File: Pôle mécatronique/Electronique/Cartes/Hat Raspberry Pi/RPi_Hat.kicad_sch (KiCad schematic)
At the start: 9 parts, among them J1 Conn_02x03_Odd_Even, U1 XBee, U2 MCP25625-x-SS, Y1 8MHz

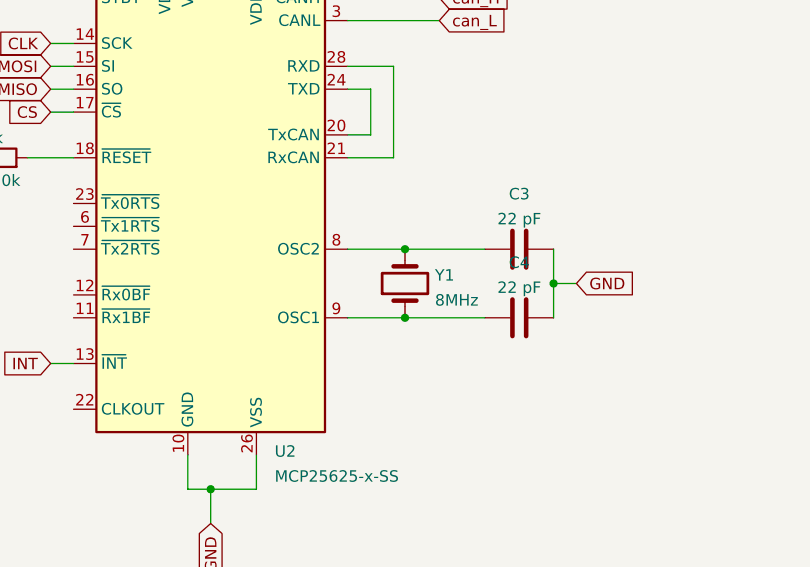
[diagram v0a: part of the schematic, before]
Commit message: Update HAT + Commande
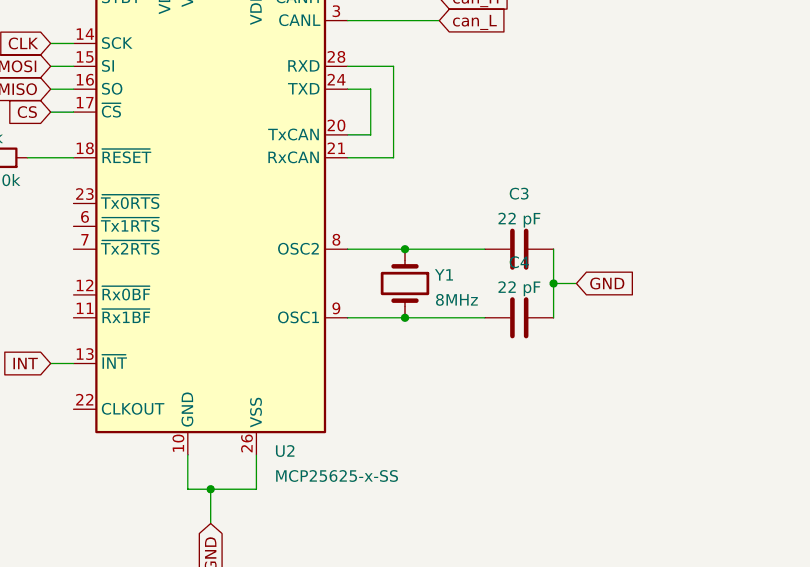
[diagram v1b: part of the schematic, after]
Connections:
- net at C4.1, U2.9 (OSC1): now also Y1.2; no longer Y1.1
- net at C3.1, U2.8 (OSC2): now also Y1.1; no longer Y1.2
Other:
- moved on the sheet: Y1
